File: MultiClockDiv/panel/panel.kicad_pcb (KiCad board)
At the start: 2 copper layers, 40.6 x 128.5 mm, 15 parts

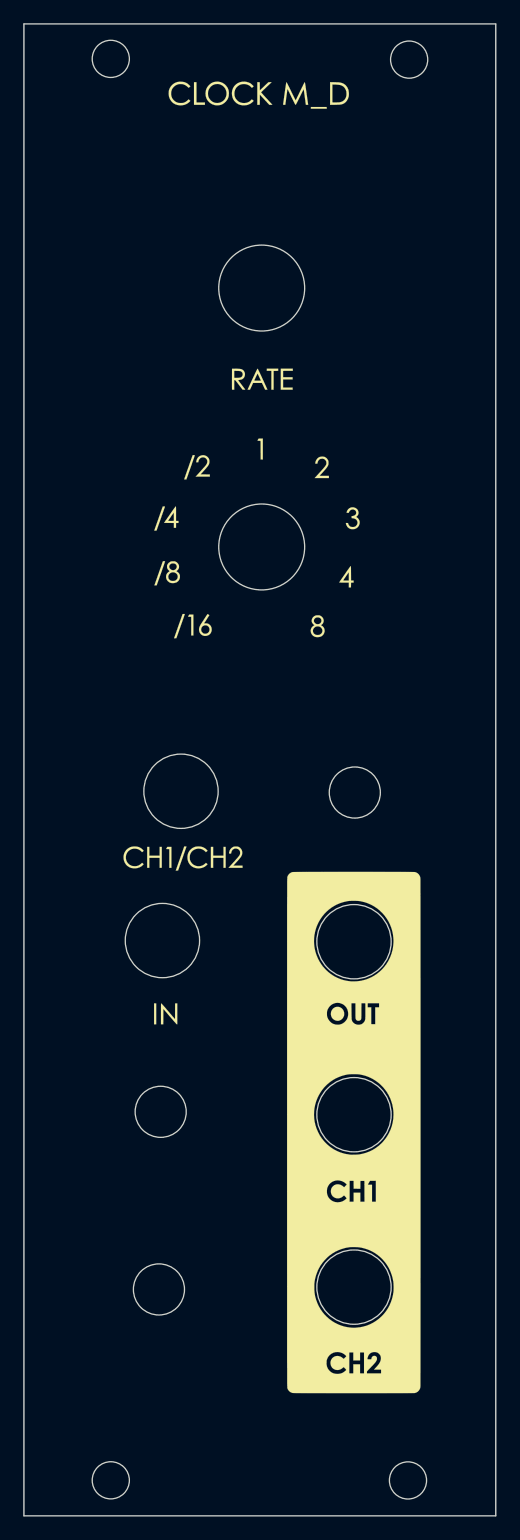
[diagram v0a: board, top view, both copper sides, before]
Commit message: correct
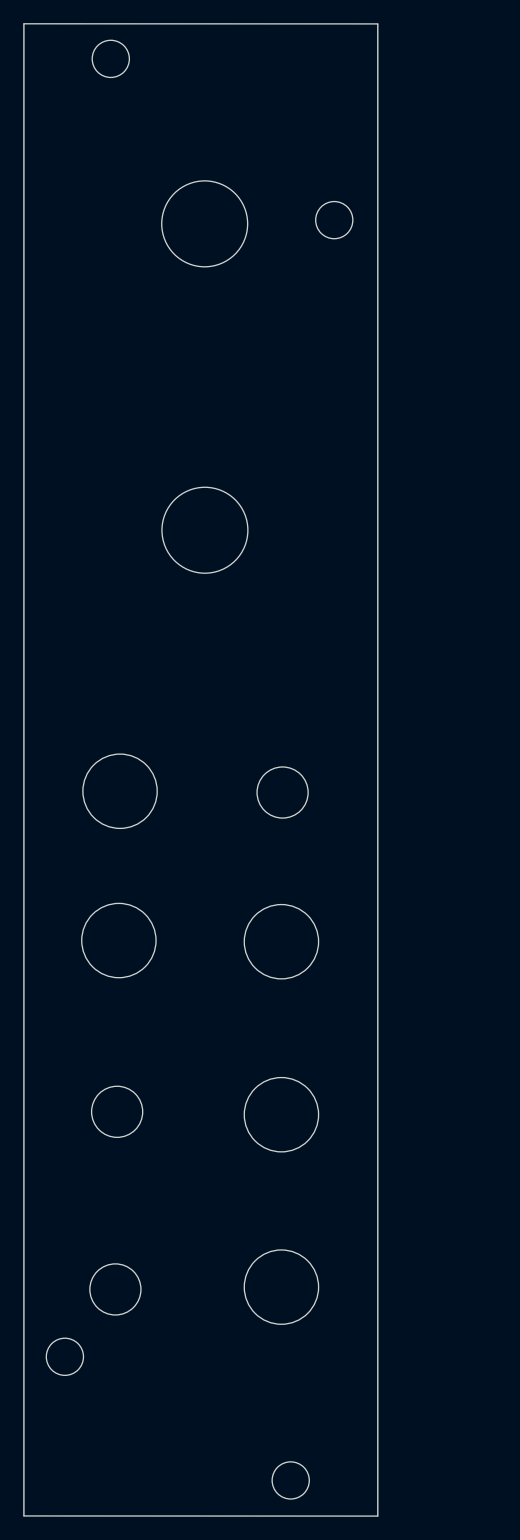
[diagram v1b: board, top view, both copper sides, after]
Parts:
- removed G***: LOGO, logo:silk13
- removed the H5 at (58.3, 153.3)
- removed the H5 at (58.4, 30.9)
- added ?: , , F.Cu at (93.3, 88.0)
- added ?: , , F.Cu at (87.4, 45.5)
- added ?: , , F.Cu at (107.0, 60.9)
- added H5: MountingHole, MountingHole:MountingHole_3.2mm_M3, F.Cu at (28.8, 142.7)
- added H5: MountingHole, MountingHole:MountingHole_3.2mm_M3, F.Cu at (48.2, 153.3)
- moved H6 110.2 mm to (52.0, 44.8)
- moved H12 7.40 mm to (40.8, 45.1)
- moved H3 6.25 mm to (47.4, 106.9)
- moved H4 6.25 mm to (47.4, 136.7)
- moved H9 6.25 mm to (47.4, 121.8)
- moved H10 6.22 mm to (47.5, 94.0)
- moved H2 5.25 mm to (33.5, 93.9)
- moved H11 5.10 mm to (40.8, 71.5)
- moved H1 3.75 mm to (33.4, 106.8)
- moved H10 3.75 mm to (33.1, 136.8)
- moved H10 3.75 mm to (33.2, 121.5)
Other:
- board size 40.6 x 128.5 mm -> 30.5 x 128.5 mm
